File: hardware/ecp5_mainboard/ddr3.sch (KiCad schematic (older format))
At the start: 55 parts, among them U23 AS4C256M16D3, U24 AS4C256M16D3, U25 TPS51200DRC

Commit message: hardware/mainboard: Assign some footprints
Signed-off-by: David Shah <dave@ds0.me>
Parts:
- C174, C176, C177, C178, C180: footprint (none) -> Capacitor_SMD:C_0805_2012Metric
- C175, C179, C181, C185, C186, C187, C188, C189, C190, C191, C192, C193, C194, C195, C196, C197, C198, C199, C200, C201, C202, C203, C204, C205, C206, C207, C208, C209, C210, C211, C212: footprint (none) -> Capacitor_SMD:C_0402_1005Metric
- C182, C183, C184: footprint (none) -> Capacitor_SMD:C_0603_1608Metric
- R75, R76, R77, R78, R79, R80, R81: footprint (none) -> Resistor_SMD:R_0402_1005Metric
- RN16, RN17, RN18, RN19, RN20, RN21: footprint (none) -> Resistor_SMD:R_Array_Convex_4x0402
- U23, U24: footprint (none) -> Package_BGA:BGA-96_9.0x13.0mm_Layout2x3x16_P0.8mm

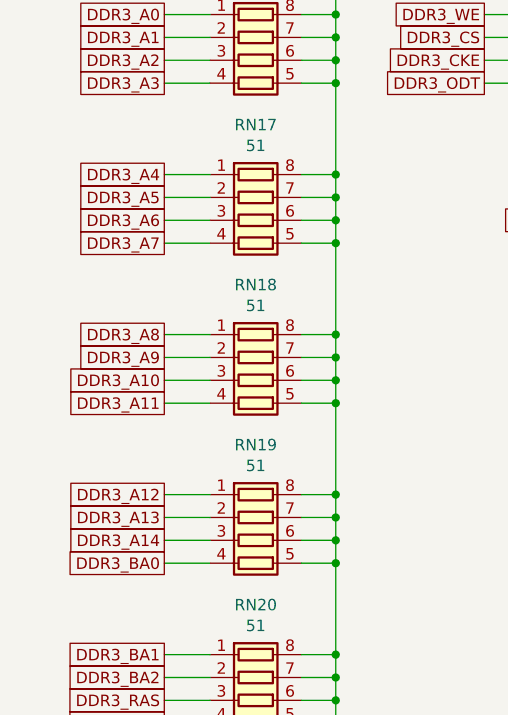
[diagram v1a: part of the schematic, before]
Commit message: hardware/mainboard: More DDR3 address routing
Signed-off-by: David Shah <dave@ds0.me>
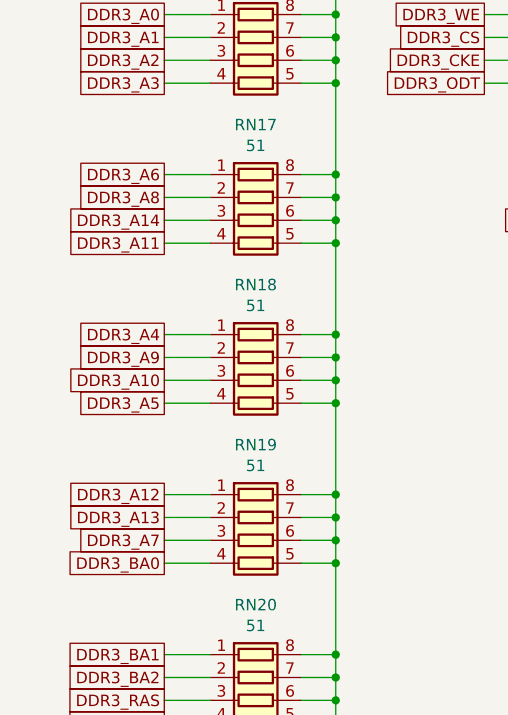
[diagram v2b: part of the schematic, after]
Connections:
- net DDR3_A11: now also RN17.4 (R4.1); no longer RN18.4 (R4.1)
- net DDR3_A14: now also RN17.3 (R3.1); no longer RN19.3 (R3.1)
- net DDR3_A4: now also RN18.1 (R1.1); no longer RN17.1 (R1.1)
- net DDR3_A5: now also RN18.4 (R4.1); no longer RN17.2 (R2.1)
- net DDR3_A6: now also RN17.1 (R1.1); no longer RN17.3 (R3.1)
- net DDR3_A7: now also RN19.3 (R3.1); no longer RN17.4 (R4.1)
- net DDR3_A8: now also RN17.2 (R2.1); no longer RN18.1 (R1.1)
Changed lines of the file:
@@
 Text GLabel 3600 8100 0    50   UnSpc ~ 0
 DDR3_A3
+Text GLabel 3600 9200 0    50   UnSpc ~ 0
+DDR3_A4
+Text GLabel 3600 9500 0    50   UnSpc ~ 0
+DDR3_A5
 Text GLabel 3600 8500 0    50   UnSpc ~ 0
-DDR3_A4
+DDR3_A6
+Text GLabel 3600 10100 0    50   UnSpc ~ 0
+DDR3_A7
 Text GLabel 3600 8600 0    50   UnSpc ~ 0
-DDR3_A5
-Text GLabel 3600 8700 0    50   UnSpc ~ 0
-DDR3_A6
-Text GLabel 3600 8800 0    50   UnSpc ~ 0
-DDR3_A7
-Text GLabel 3600 9200 0    50   UnSpc ~ 0
 DDR3_A8
 Text GLabel 3600 9300 0    50   UnSpc ~ 0
@@
 Text GLabel 3600 9400 0    50   UnSpc ~ 0
 DDR3_A10
-Text GLabel 3600 9500 0    50   UnSpc ~ 0
+Text GLabel 3600 8800 0    50   UnSpc ~ 0
 DDR3_A11
 Text GLabel 3600 9900 0    50   UnSpc ~ 0
@@
 Text GLabel 3600 10000 0    50   UnSpc ~ 0
 DDR3_A13
-Text GLabel 3600 10100 0    50   UnSpc ~ 0
+Text GLabel 3600 8700 0    50   UnSpc ~ 0
 DDR3_A14
 Wire Wire Line
@@
 	3800 8100 3600 8100
 Wire Wire Line
+	3600 9200 3800 9200
+Wire Wire Line
+	3600 9500 3800 9500
+Wire Wire Line
 	3600 8500 3800 8500
 Wire Wire Line
+	3600 10100 3800 10100
+Wire Wire Line
 	3600 8600 3800 8600
-Wire Wire Line
-	3600 8700 3800 8700
-Wire Wire Line
-	3600 8800 3800 8800
-Wire Wire Line
-	3600 9200 3800 9200
 Wire Wire Line
 	3600 9300 3800 9300
@@
 	3600 9400 3800 9400
 Wire Wire Line
-	3600 9500 3800 9500
+	3600 8800 3800 8800
 Wire Wire Line
 	3600 9900 3800 9900
@@
 	3600 10000 3800 10000
 Wire Wire Line
-	3600 10100 3800 10100
+	3600 8700 3800 8700
 Text GLabel 3600 10200 0    50   UnSpc ~ 0
 DDR3_BA0

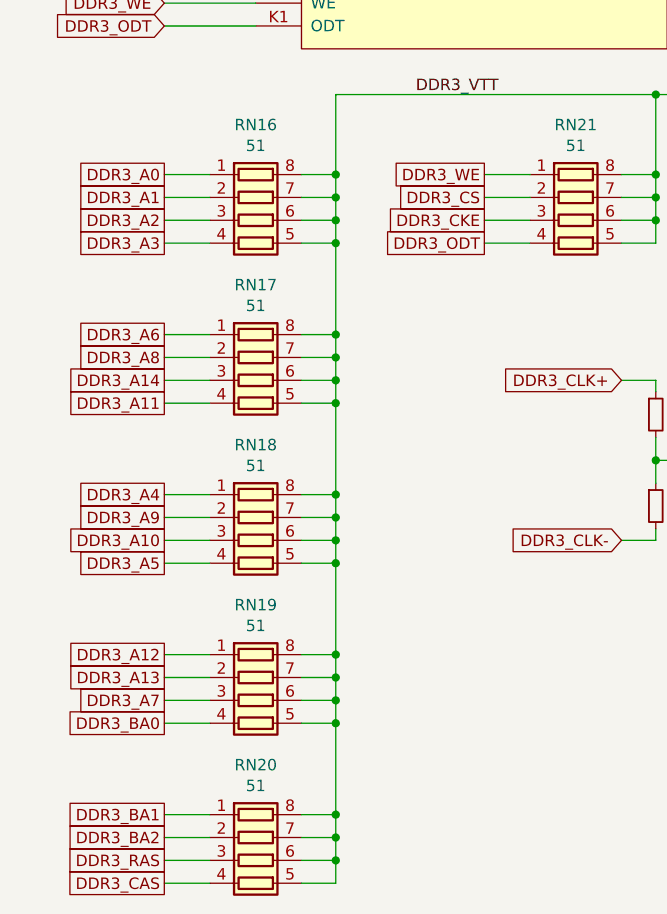
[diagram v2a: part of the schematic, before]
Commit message: hardware/mainboard: Finish DDR3 CA routing inc termination
Signed-off-by: David Shah <dave@ds0.me>
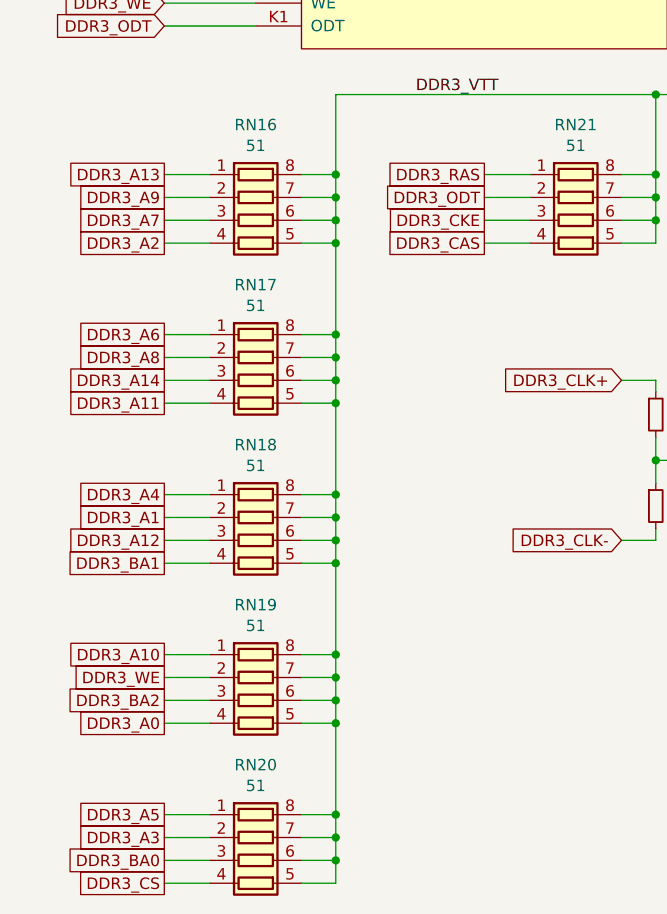
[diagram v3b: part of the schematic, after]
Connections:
- net DDR3_A0: now also RN19.4 (R4.1); no longer RN16.1 (R1.1)
- net DDR3_A1: now also RN18.2 (R2.1); no longer RN16.2 (R2.1)
- net DDR3_A10: now also RN19.1 (R1.1); no longer RN18.3 (R3.1)
- net DDR3_A12: now also RN18.3 (R3.1); no longer RN19.1 (R1.1)
- net DDR3_A13: now also RN16.1 (R1.1); no longer RN19.2 (R2.1)
- net DDR3_A2: now also RN16.4 (R4.1); no longer RN16.3 (R3.1)
- net DDR3_A3: now also RN20.2 (R2.1); no longer RN16.4 (R4.1)
- net DDR3_A5: now also RN20.1 (R1.1); no longer RN18.4 (R4.1)
- net DDR3_A7: now also RN16.3 (R3.1); no longer RN19.3 (R3.1)
- net DDR3_A9: now also RN16.2 (R2.1); no longer RN18.2 (R2.1)
- net DDR3_BA0: now also RN20.3 (R3.1); no longer RN19.4 (R4.1)
- net DDR3_BA1: now also RN18.4 (R4.1); no longer RN20.1 (R1.1)
- net DDR3_BA2: now also RN19.3 (R3.1); no longer RN20.2 (R2.1)
- net DDR3_CAS: now also RN21.4 (R4.1); no longer RN20.4 (R4.1)
- net DDR3_CS: now also RN20.4 (R4.1); no longer RN21.2 (R2.1)
- net DDR3_ODT: now also RN21.2 (R2.1); no longer RN21.4 (R4.1)
- net DDR3_RAS: now also RN21.1 (R1.1); no longer RN20.3 (R3.1)
- net DDR3_WE: now also RN19.2 (R2.1); no longer RN21.1 (R1.1)
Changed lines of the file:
@@
 	0    1    1    0
 $EndComp
-Text GLabel 3600 7800 0    50   UnSpc ~ 0
+Text GLabel 3600 10200 0    50   UnSpc ~ 0
 DDR3_A0
-Text GLabel 3600 7900 0    50   UnSpc ~ 0
+Text GLabel 3600 9300 0    50   UnSpc ~ 0
 DDR3_A1
-Text GLabel 3600 8000 0    50   UnSpc ~ 0
+Text GLabel 3600 8100 0    50   UnSpc ~ 0
 DDR3_A2
-Text GLabel 3600 8100 0    50   UnSpc ~ 0
+Text GLabel 3600 10700 0    50   UnSpc ~ 0
 DDR3_A3
 Text GLabel 3600 9200 0    50   UnSpc ~ 0
 DDR3_A4
-Text GLabel 3600 9500 0    50   UnSpc ~ 0
+Text GLabel 3600 10600 0    50   UnSpc ~ 0
 DDR3_A5
 Text GLabel 3600 8500 0    50   UnSpc ~ 0
 DDR3_A6
-Text GLabel 3600 10100 0    50   UnSpc ~ 0
+Text GLabel 3600 8000 0    50   UnSpc ~ 0
 DDR3_A7
 Text GLabel 3600 8600 0    50   UnSpc ~ 0
 DDR3_A8
-Text GLabel 3600 9300 0    50   UnSpc ~ 0
+Text GLabel 3600 7900 0    50   UnSpc ~ 0
 DDR3_A9
-Text GLabel 3600 9400 0    50   UnSpc ~ 0
+Text GLabel 3600 9900 0    50   UnSpc ~ 0
 DDR3_A10
 Text GLabel 3600 8800 0    50   UnSpc ~ 0
 DDR3_A11
-Text GLabel 3600 9900 0    50   UnSpc ~ 0
+Text GLabel 3600 9400 0    50   UnSpc ~ 0
 DDR3_A12
-Text GLabel 3600 10000 0    50   UnSpc ~ 0
+Text GLabel 3600 7800 0    50   UnSpc ~ 0
 DDR3_A13
 Text GLabel 3600 8700 0    50   UnSpc ~ 0
 DDR3_A14
 Wire Wire Line
-	3600 7800 3800 7800
+	3600 10200 3800 10200
 Wire Wire Line
-	3800 7900 3600 7900
-Wire Wire Line
-	3800 8000 3600 8000
+	3800 9300 3600 9300
 Wire Wire Line
 	3800 8100 3600 8100
 Wire Wire Line
+	3800 10700 3600 10700
+Wire Wire Line
 	3600 9200 3800 9200
 Wire Wire Line
-	3600 9500 3800 9500
+	3600 10600 3800 10600
 Wire Wire Line
 	3600 8500 3800 8500
 Wire Wire Line
-	3600 10100 3800 10100
+	3600 8000 3800 8000
 Wire Wire Line
 	3600 8600 3800 8600
 Wire Wire Line
-	3600 9300 3800 9300
+	3600 7900 3800 7900
+Wire Wire Line
+	3600 9900 3800 9900
+Wire Wire Line
+	3600 8800 3800 8800
 Wire Wire Line
 	3600 9400 3800 9400
 Wire Wire Line
-	3600 8800 3800 8800
-Wire Wire Line
-	3600 9900 3800 9900
-Wire Wire Line
-	3600 10000 3800 10000
+	3600 7800 3800 7800
 Wire Wire Line
 	3600 8700 3800 8700
-Text GLabel 3600 10200 0    50   UnSpc ~ 0
+Text GLabel 3600 10800 0    50   UnSpc ~ 0
 DDR3_BA0
-Text GLabel 3600 10600 0    50   UnSpc ~ 0
+Text GLabel 3600 9500 0    50   UnSpc ~ 0
 DDR3_BA1
-Text GLabel 3600 10700 0    50   UnSpc ~ 0
+Text GLabel 3600 10100 0    50   UnSpc ~ 0
 DDR3_BA2
 Wire Wire Line
-	3600 10200 3800 10200
+	3600 10800 3800 10800
 Wire Wire Line
-	3800 10600 3600 10600
+	3800 9500 3600 9500
 Wire Wire Line
-	3600 10700 3800 10700
-Text GLabel 3600 10800 0    50   UnSpc ~ 0
+	3600 10100 3800 10100
+Text GLabel 5000 7800 0    50   UnSpc ~ 0
 DDR3_RAS
-Text GLabel 3600 10900 0    50   UnSpc ~ 0
+Text GLabel 5000 8100 0    50   UnSpc ~ 0
 DDR3_CAS
 Wire Wire Line
-	3600 10900 3800 10900
+	5000 8100 5200 8100
 Wire Wire Line
-	3800 10800 3600 10800
+	5200 7800 5000 7800
 $Comp
 L Device:R_Pack04 RN21
@@
 	0    1    1    0
 $EndComp
-Text GLabel 5000 7800 0    50   UnSpc ~ 0
+Text GLabel 3600 10000 0    50   UnSpc ~ 0
 DDR3_WE
-Text GLabel 5000 7900 0    50   UnSpc ~ 0
+Text GLabel 3600 10900 0    50   UnSpc ~ 0
 DDR3_CS
 Wire Wire Line
-	5200 7800 5000 7800
+	3800 10000 3600 10000
+Wire Wire Line
+	3600 10900 3800 10900
+Text GLabel 5000 8000 0    50   UnSpc ~ 0
+DDR3_CKE
+Text GLabel 5000 7900 0    50   UnSpc ~ 0
+DDR3_ODT
 Wire Wire Line
 	5000 7900 5200 7900
-Text GLabel 5000 8000 0    50   UnSpc ~ 0
-DDR3_CKE
-Text GLabel 5000 8100 0    50   UnSpc ~ 0
-DDR3_ODT
-Wire Wire Line
-	5000 8100 5200 8100
 Wire Wire Line
 	5200 8000 5000 8000

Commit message: hardware/mainboard: BoM fixes, add USB power option
Signed-off-by: David Shah <dave@ds0.me>
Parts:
- C182: footprint Capacitor_SMD:C_0603_1608Metric -> Capacitor_SMD:C_0805_2012Metric
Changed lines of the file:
@@
 EESchema Schematic File Version 4
 LIBS:ecp5_mainboard-cache
-EELAYER 26 0
+EELAYER 29 0
 EELAYER END
 $Descr A3 16535 11693
@@
 F 0 "C182" H 9642 7646 50  0000 L CNN
 F 1 "10µ" H 9642 7555 50  0000 L CNN
-F 2 "Capacitor_SMD:C_0603_1608Metric" H 9550 7600 50  0001 C CNN
+F 2 "Capacitor_SMD:C_0805_2012Metric" H 9550 7600 50  0001 C CNN
 F 3 "~" H 9550 7600 50  0001 C CNN
 	1    9550 7600
